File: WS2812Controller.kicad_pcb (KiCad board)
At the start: 2 copper layers, 54.9 x 53.8 mm, 19 parts, among them J1 USB_B_Micro, J2 Conn_01x05_Male, J3 Conn_01x03, SW1 SW_Reset, SW2 SW_GPIO0, U1 AMS1117-3.3, U2 ESP-12F

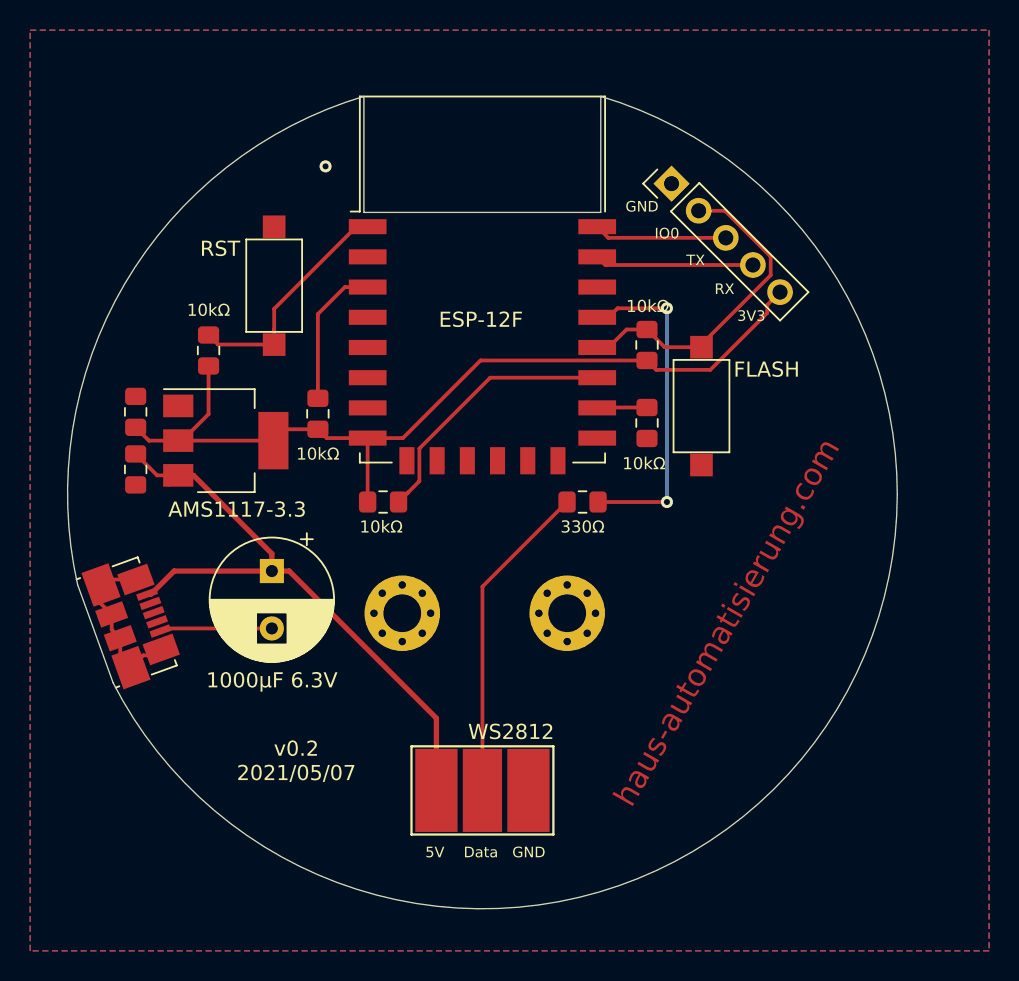
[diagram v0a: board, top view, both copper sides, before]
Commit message: New layout
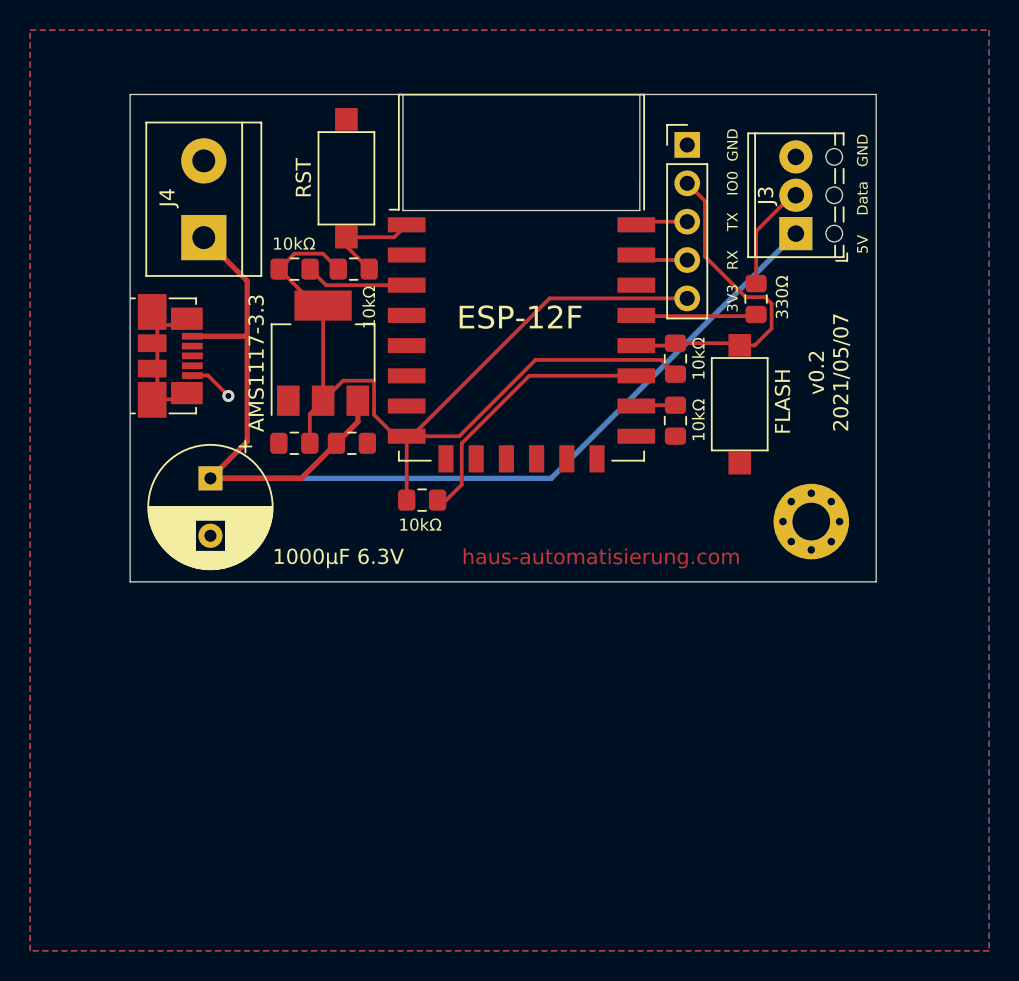
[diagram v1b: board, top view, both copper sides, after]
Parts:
- removed the REF** at (128.8, 104.6)
- added J4: Conn_01x02_Male, TerminalBlock:TerminalBlock_bornier-2_P5.08mm, F.Cu at (115.6, 79.8)
- J3: footprint halibs:SolderPads3 -> TerminalBlock_Phoenix:TerminalBlock_Phoenix_MPT-0,5-3-2.54_1x03_P2.54mm_Horizontal
- moved J3 38.3 mm to (154.8, 79.5), turned to 90 degrees
- moved R6 17.7 mm to (152.2, 83.8), turned to 270 degrees
- moved J1 17.7 mm to (113.4, 87.6), turned to 270 degrees
- moved REF** 17.3 mm to (155.9, 98.6)
- moved C1 14.4 mm to (125.4, 93.4), turned to 0 degrees
- moved R3 11.0 mm to (125.6, 81.9), turned to 0 degrees
- moved C2 10.7 mm to (121.6, 93.4), turned to 180 degrees
- moved R1 9.70 mm to (121.6, 81.9), turned to 0 degrees
- moved U1 8.66 mm to (123.5, 87.4), turned to 90 degrees
- moved SW1 8.57 mm to (125.1, 75.8)
- moved C3 7.36 mm to (116.1, 95.7)
- moved J2 2.76 mm to (147.6, 73.6), turned to 0 degrees
- moved G*** 2.59 mm to (136.7, 90.1)
- moved U2 2.59 mm to (136.7, 82.4)
- moved R4 2.59 mm to (130.1, 97.2)
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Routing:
- net +5V: track 42.4 -> 80.0 mm
- net +3V3: track 58.6 -> 73.9 mm
- net GPIO4: track 22.3 -> 8.00 mm, vias 2 -> 0
- net Net-(J3-Pad2): track 21.6 -> 7.44 mm
- net /RST: track 15.4 -> 7.83 mm
- net RX: track 10.5 -> 3.51 mm
- net TX: track 8.82 -> 3.46 mm
- net GND: track 6.90 -> 2.95 mm
- net /EN: track 9.62 -> 6.84 mm
- net Net-(R2-Pad1): track 3.31 -> 2.62 mm
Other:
- board size 54.9 x 53.8 mm -> 49.4 x 32.3 mm
- board text added: "+"
- board text added: "-"
- board text removed: "WS2812"
